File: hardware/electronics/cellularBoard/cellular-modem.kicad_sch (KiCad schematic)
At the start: 25 parts, among them Q1 DMG1013TQ-7, U2 LEXI-R520, U3 LM51571-Q1, U4 OPA344

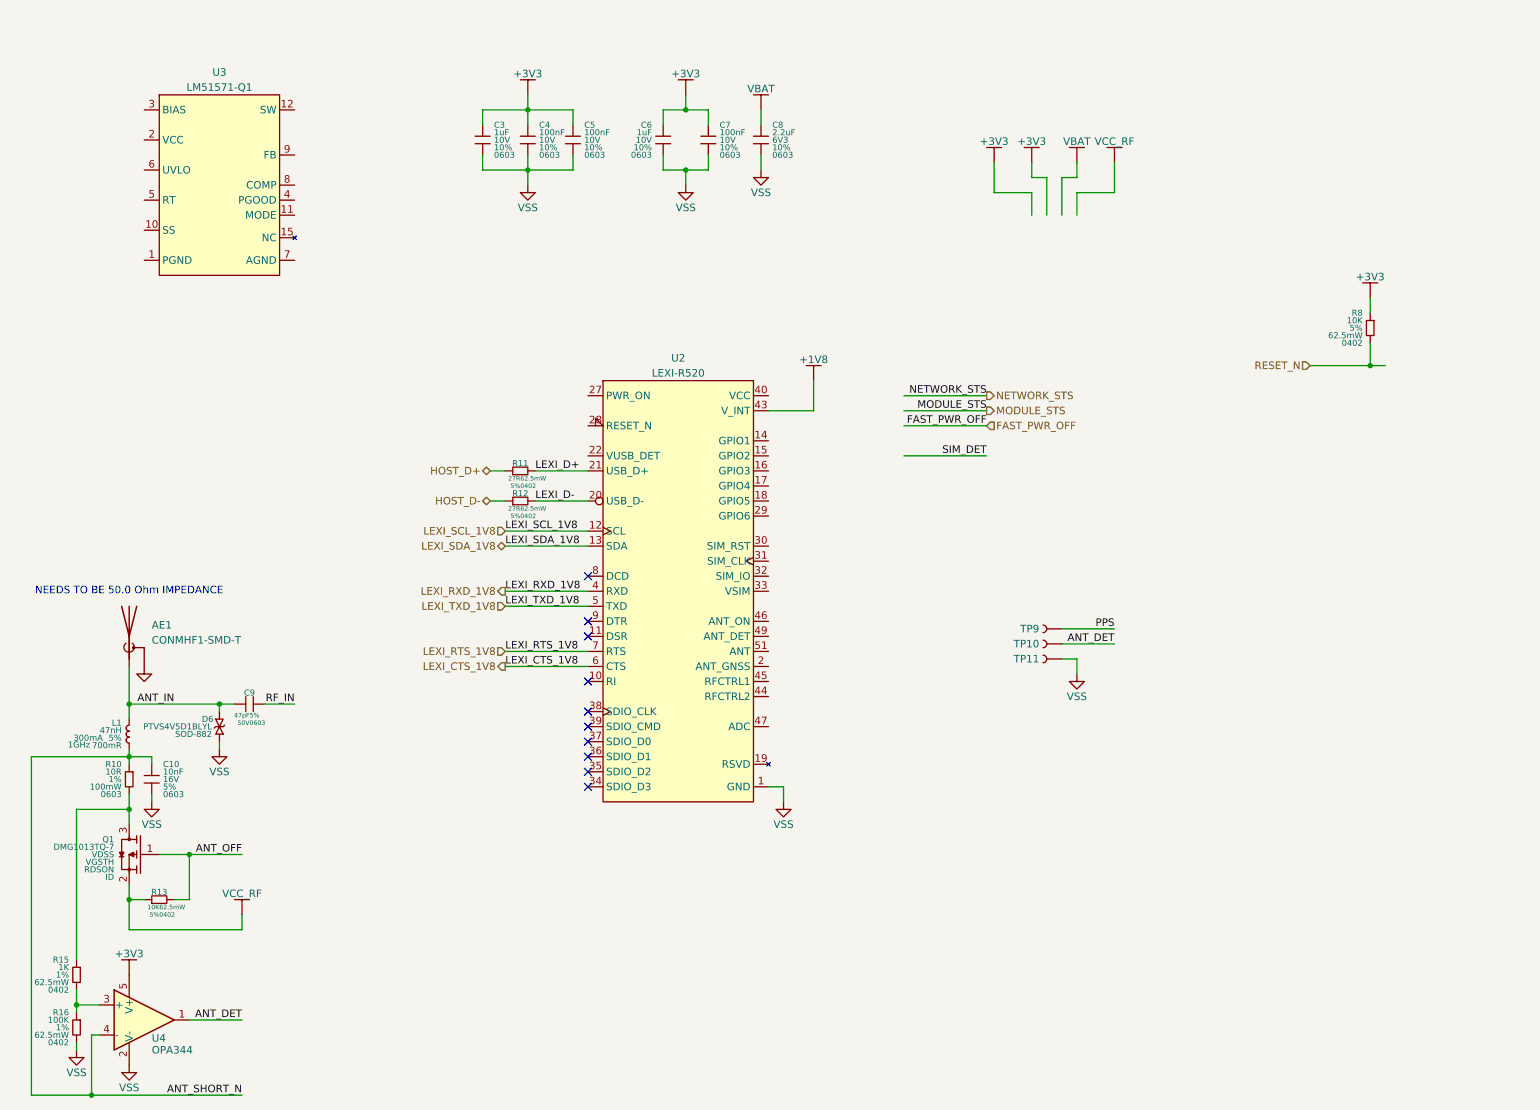
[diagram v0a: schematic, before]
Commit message: finished schematic
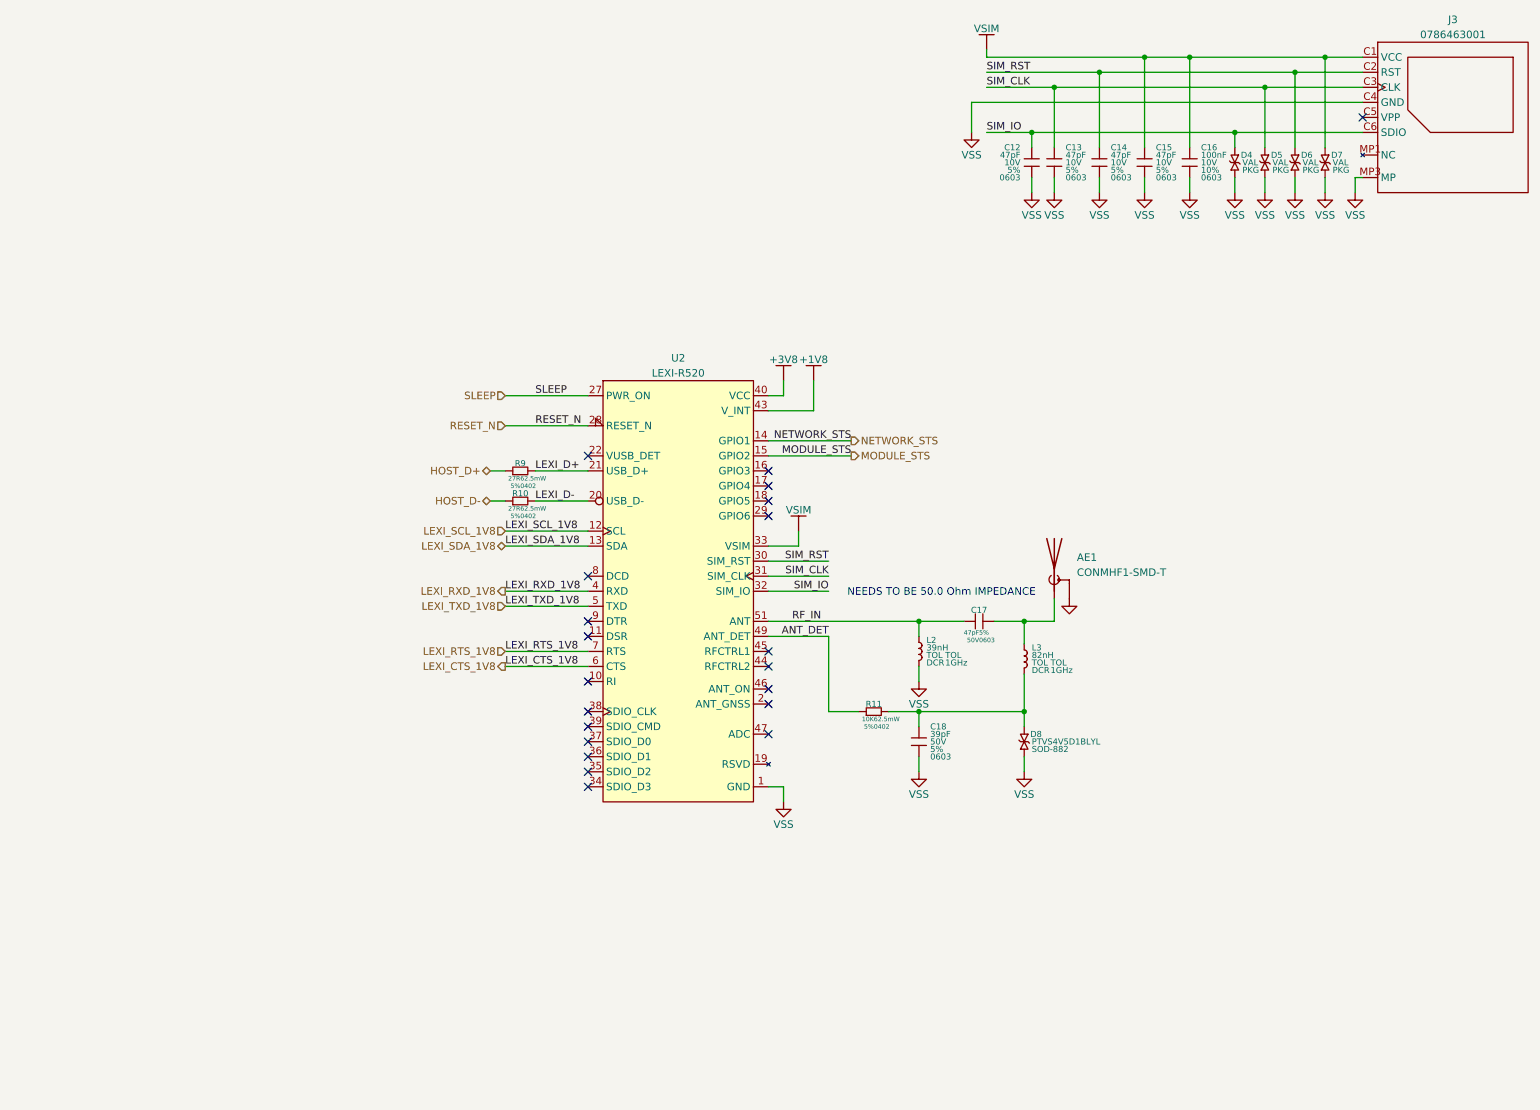
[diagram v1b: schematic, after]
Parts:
- removed C10: 10nF, lib_fp:MLCC0603, symbol lib_sch:C
- removed C3, C6: 1uF, lib_fp:MLCC0603, symbol lib_sch:C
- removed C4, C5, C7: 100nF, lib_fp:MLCC0603, symbol lib_sch:C
- removed C8: 2.2uF, lib_fp:MLCC0603, symbol lib_sch:C
- removed C9: 47pF, lib_fp:MLCC0603, symbol lib_sch:C_horizontal
- removed L1: 47nH, lib_fp:L_0402, symbol lib_sch:L
- removed Q1: DMG1013TQ-7, lib_fp:SOT23-3P50_160X160X75L22X22N, symbol lib_sch:PMOS_DGS
- removed R10: 10R, lib_fp:CRCW0603, symbol lib_sch:R
- removed R13: 10K, lib_fp:CRCW0402, symbol lib_sch:R_horizontal
- removed R15: 1K, lib_fp:CRCW0402, symbol lib_sch:R
- removed R16: 100K, lib_fp:CRCW0402, symbol lib_sch:R
- removed R8: 10K, lib_fp:CRCW0402, symbol lib_sch:R
- removed TP10, TP11, TP9: ~, lib_fp:TP_1mm, symbol lib_sch:Testpoint
- removed U3: LM51571-Q1, symbol lib_sch:LM51571-Q1
- removed U4: OPA344, lib_fp:SOT23-5P95_280X300X110L40X38N, symbol lib_sch:TS391
- added C12, C13, C14, C15: 47pF, lib_fp:MLCC0603, symbol lib_sch:C
- added C16: 100nF, lib_fp:MLCC0603, symbol lib_sch:C
- added C17: 47pF, lib_fp:MLCC0603, symbol lib_sch:C_horizontal
- added C18: 39pF, lib_fp:MLCC0603, symbol lib_sch:C
- added D4, D5, D7: VAL, lib_fp:SOD882, symbol lib_sch:D_TVS
- added D8: PTVS4V5D1BLYL, lib_fp:SOD882, symbol lib_sch:D_TVS
- added J3: 0786463001, symbol lib_sch:SIM_Card
- added L2: 39nH, symbol lib_sch:L
- added L3: 82nH, symbol lib_sch:L
- added R11: 10K, lib_fp:CRCW0402, symbol lib_sch:R_horizontal
- D6: value PTVS4V5D1BLYL -> VAL; Package SOD-882 -> PKG
- renumbered R12 to R10, R11 to R9
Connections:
- net ANT_DET: now also U2.49 (ANT_DET), R11.1
- net MODULE_STS: now also U2.15 (GPIO2)
- net NETWORK_STS: now also U2.14 (GPIO1)
- net RESET_N: now also U2.28 (RESET_N)
- net RF_IN: now also U2.51 (ANT), C17.1, L2.1
- net VSS: now also C12.2, C13.2, C14.2, C15.2, C16.2, C18.2, D4.1, D5.1, D7.1, D8.1, J3.C4 (GND), J3.MP3 (MP), J3.MP4 (MP), J3.MP5 (MP), J3.MP6 (MP), J3.MP7 (MP), J3.MP8 (MP), L2.2
- net SLEEP: now reaches U2.27 (PWR_ON)
- net SIM_RST: now reaches U2.30 (SIM_RST)
- net SIM_RST: now also D6.2, C14.1, J3.C2 (RST)
- net SIM_CLK: now reaches U2.31 (SIM_CLK)
- net SIM_CLK: now also C13.1, D5.2, J3.C3 (CLK)
- net SIM_IO: now reaches U2.32 (SIM_IO)
- net SIM_IO: now also C12.1, D4.2, J3.C6 (SDIO)
- net VSIM: now reaches U2.33 (VSIM)
- net VSIM: now also C15.1, C16.1, D7.2, J3.C1 (VCC)
- net ANT_IN: no longer names the net of AE1.1 (A)
- net ANT_IN: now also C17.2, L3.1; no longer D6.2
- net VCC renamed +3V8
- new net: J3.MP1 (NC), J3.MP2 (NC)
- new net: C18.1, D8.2, L3.2, R11.2
- no-connect marks 10 -> 21
